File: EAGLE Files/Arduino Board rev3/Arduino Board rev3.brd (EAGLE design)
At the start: 40 x 40 mm, 6 parts

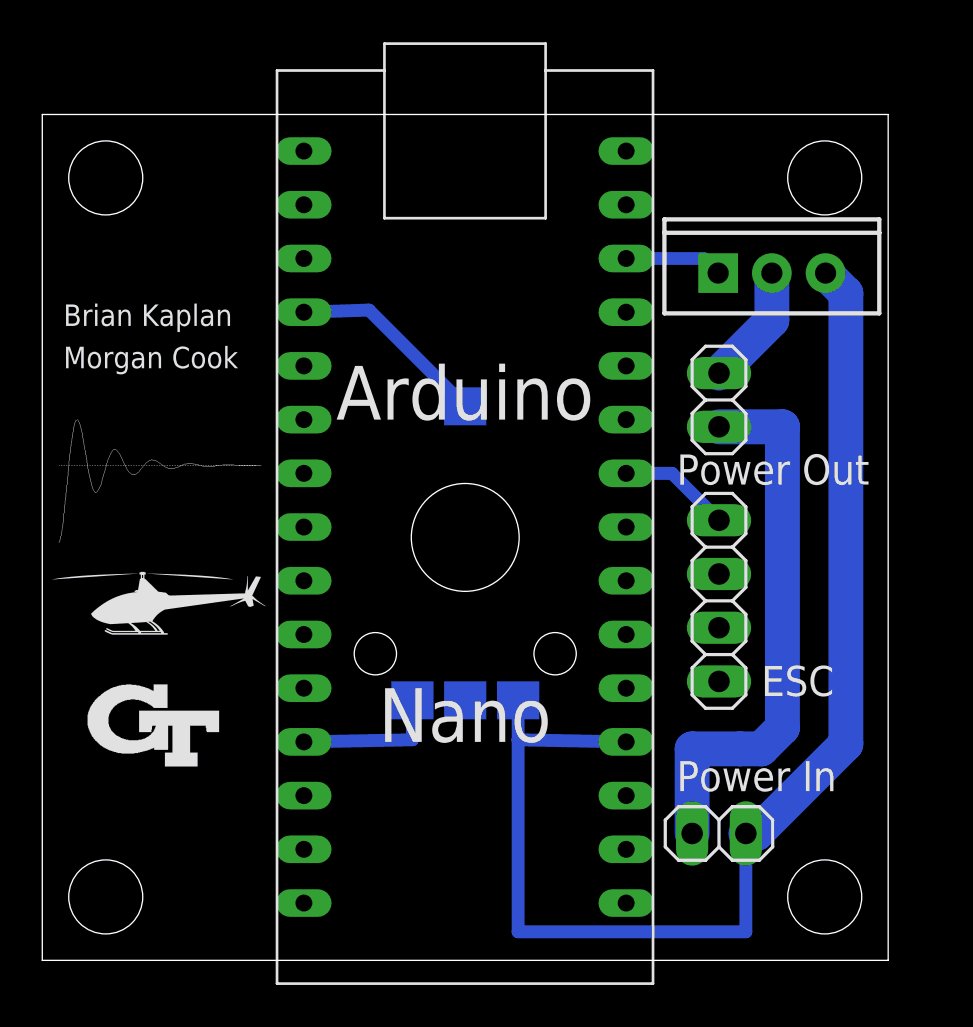
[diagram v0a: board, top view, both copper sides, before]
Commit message: Finalized PCB designs and generated Gerber files for manufacturing
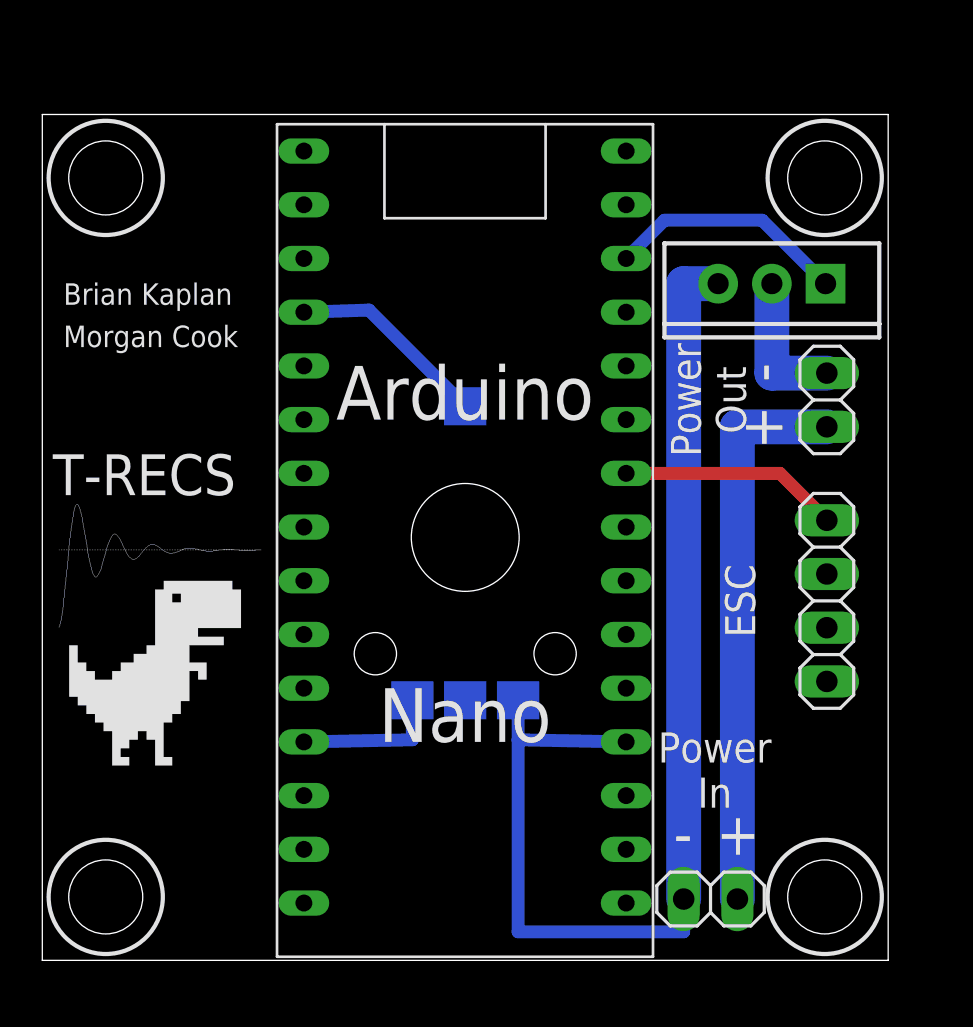
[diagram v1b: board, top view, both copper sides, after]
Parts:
- moved ESC 5.10 mm to (37.1, 17.0)
- moved POWER_OUT 5.10 mm to (37.1, 26.5)
- moved POWER_IN 3.13 mm to (31.6, 2.90), turned to 180 degrees
- moved MOSFET 0.50 mm to (34.5, 32.0), turned to 180 degrees
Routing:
- net DRIVE: track 4.64 -> 11.4 mm
- net ESC: track 5.31 -> 10.4 mm
- net GND: track 60.6 -> 56.2 mm
- net N$3: track 5.77 -> 6.83 mm
- net 12V: track 25.9 -> 26.6 mm
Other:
- board text added: "+"
- board text added: "-"
- board text added: "T-RECS"
